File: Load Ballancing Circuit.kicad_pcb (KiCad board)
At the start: 2 copper layers, 39.4 x 46.6 mm, 12 parts, among them J1 1757284, U1 LTC4359HMS8#PBF, U2 LTC4359HMS8#PBF

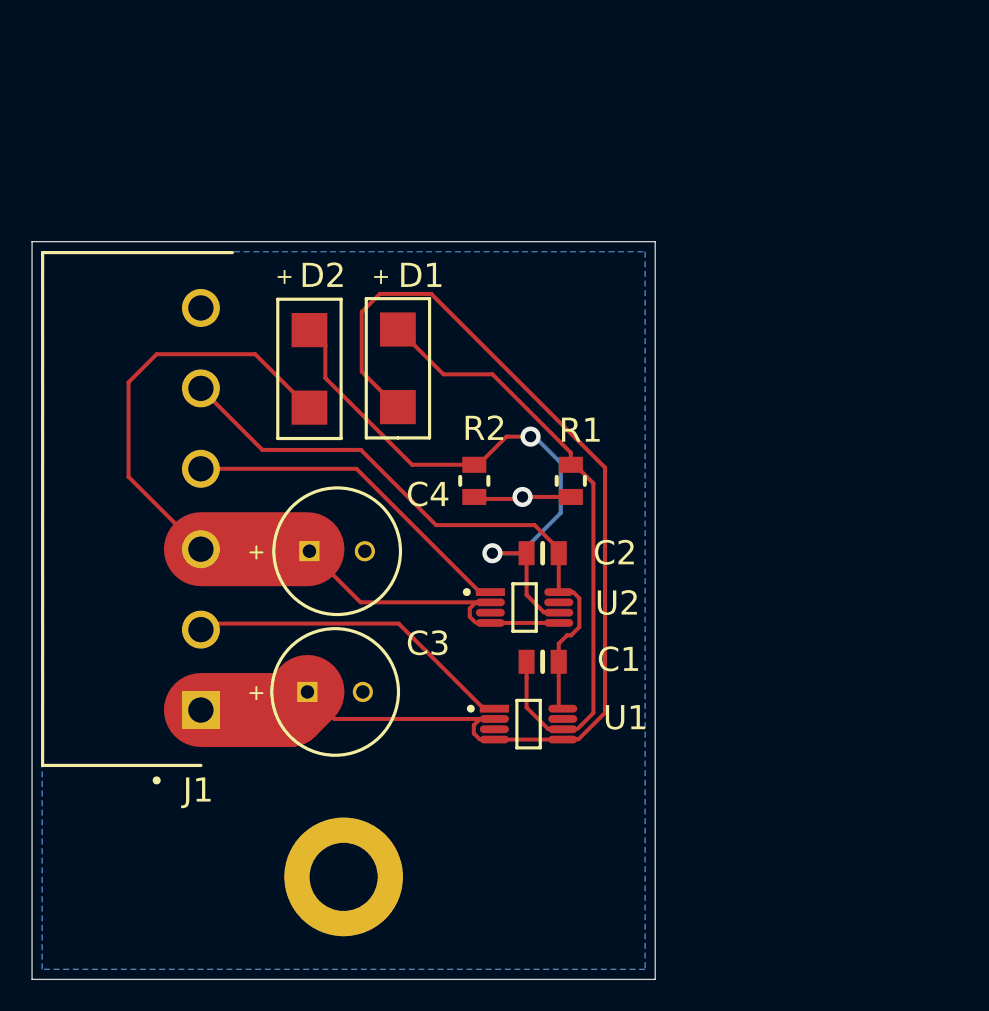
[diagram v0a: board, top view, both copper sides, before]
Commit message: added connectors and did layout
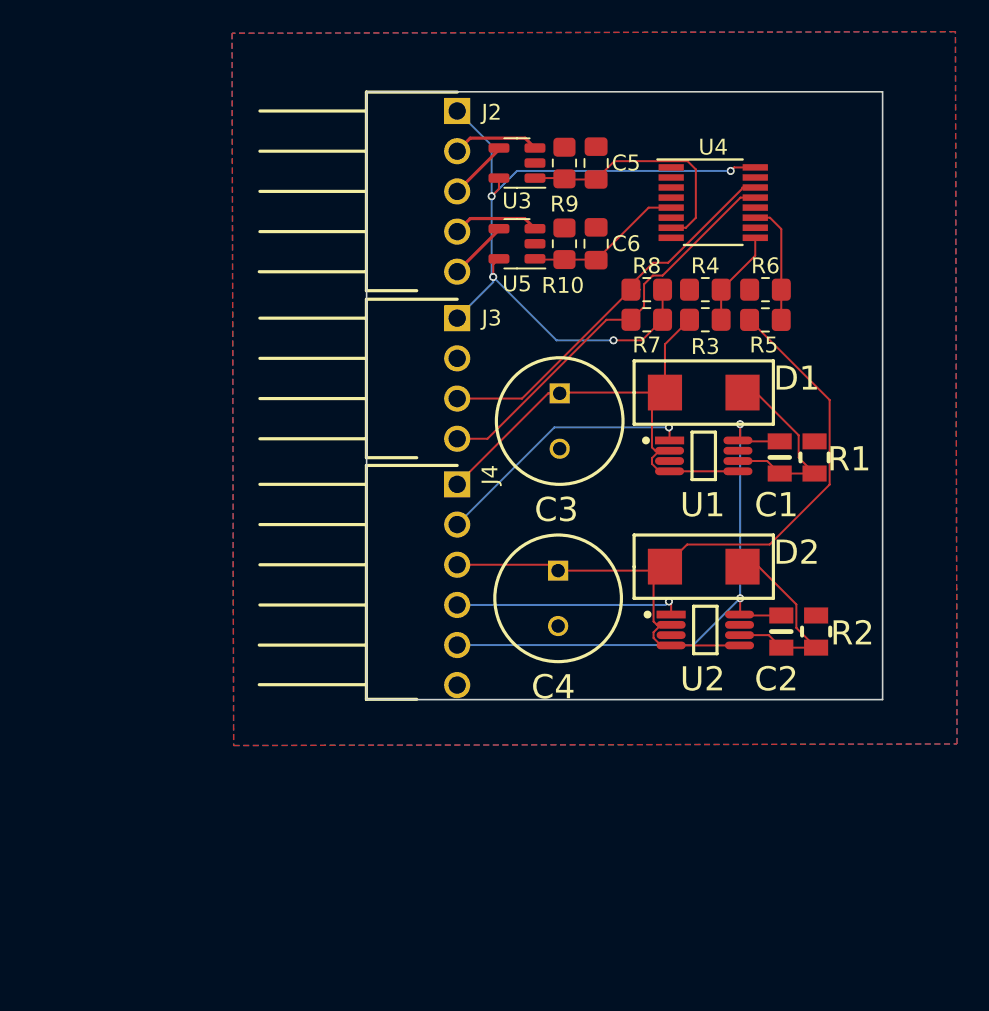
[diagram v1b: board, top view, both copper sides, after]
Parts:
- removed J1: 1757284, AltiumImport:SHDRRA6W100P0X508_1X6_3240X1200X860P
- removed REF**: MountingHole_4.3mm_M4_DIN965_Pad, AltiumImport:MountingHole_4.3mm_M4_DIN965_Pad
- added C5: 8p, Capacitor_SMD:C_0805_2012Metric_Pad1.18x1.45mm_HandSolder, F.Cu at (164.5, 76.7)
- added C6: 8p, Capacitor_SMD:C_0805_2012Metric_Pad1.18x1.45mm_HandSolder, F.Cu at (164.5, 81.8)
- added J2: 171857-0005, KK254:1718570005, F.Cu at (157.0, 72.0)
- added J3: 171857-0004, KK254:1718570004, F.Cu at (157.0, 85.1)
- added J4: 171857-0006, KK254:1718570006, F.Cu at (157.0, 95.6)
- added R10: 27k, Resistor_SMD:R_0805_2012Metric_Pad1.20x1.40mm_HandSolder, F.Cu at (162.5, 81.8)
- added R3: 10M, Resistor_SMD:R_0805_2012Metric_Pad1.20x1.40mm_HandSolder, F.Cu at (171.4, 86.6)
- added R4: 1.38M, Resistor_SMD:R_0805_2012Metric_Pad1.20x1.40mm_HandSolder, F.Cu at (171.4, 84.7)
- added R5: 10M, Resistor_SMD:R_0805_2012Metric_Pad1.20x1.40mm_HandSolder, F.Cu at (175.1, 86.6)
- added R6: 1.38M, Resistor_SMD:R_0805_2012Metric_Pad1.20x1.40mm_HandSolder, F.Cu at (175.2, 84.7)
- added R7: DNP, Resistor_SMD:R_0805_2012Metric_Pad1.20x1.40mm_HandSolder, F.Cu at (167.7, 86.6)
- added R8: DNP, Resistor_SMD:R_0805_2012Metric_Pad1.20x1.40mm_HandSolder, F.Cu at (167.7, 84.7)
- added R9: 27k, Resistor_SMD:R_0805_2012Metric_Pad1.20x1.40mm_HandSolder, F.Cu at (162.5, 76.7)
- added U3: INA139, Package_TO_SOT_SMD:SOT-23-5, F.Cu at (159.5, 76.7)
- added U4: MAX11615, Package_SO:QSOP-16_3.9x4.9mm_P0.635mm, F.Cu at (171.9, 79.2)
- added U5: INA139, Package_TO_SOT_SMD:SOT-23-5, F.Cu at (159.5, 81.8)
- moved D2 27.9 mm to (171.3, 102.2), turned to 0 degrees
- moved C3 24.7 mm to (162.2, 91.3), turned to -90 degrees
- moved R2 23.6 mm to (178.4, 106.3), turned to 180 degrees
- moved U1 20.2 mm to (171.3, 95.2)
- moved C1 19.8 mm to (176.1, 95.3), turned to 0 degrees
- moved D1 19.4 mm to (171.3, 91.2), turned to 0 degrees
- moved C2 15.9 mm to (176.2, 106.3), turned to 0 degrees
- moved C4 15.8 mm to (162.1, 102.5), turned to -90 degrees
- moved R1 15.5 mm to (178.3, 95.3), turned to 180 degrees
- moved U2 11.5 mm to (171.4, 106.2)
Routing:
- net 3V3: track 0.00 -> 49.8 mm, vias 0 -> 4
- net /V_BAT_IN_1: track 73.7 -> 33.1 mm
- net /I2C_SCL: track 0.00 -> 26.0 mm
- net /I2C_SDA: track 0.00 -> 25.9 mm
- net Net-(D1-2): track 38.5 -> 12.7 mm
- net Net-(D2-2): track 38.0 -> 12.8 mm, vias 2 -> 0
- net Net-(U4-AIN2): track 0.00 -> 15.8 mm
- net Net-(U4-AIN0): track 0.00 -> 10.0 mm
- net Net-(U4-AIN6): track 0.00 -> 7.68 mm
- net /GATE_2: track 21.5 -> 14.4 mm, vias 0 -> 1
- net Net-(U4-AIN4): track 0.00 -> 6.07 mm
- net /SNS2+: track 0.00 -> 5.52 mm
- net /SNS1+: track 0.00 -> 5.51 mm
- net GND: track 5.21 -> 0.00 mm, vias 1 -> 0
- net /GATE_1: track 20.9 -> 16.8 mm, vias 0 -> 1
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- added copper zone on F.Cu, net GND
- removed copper zone on B.Cu, net (none)
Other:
- board size 39.4 x 46.6 mm -> 32.6 x 38.4 mm
- board text removed: "+"
- board text removed: "Load Balancing Board v1.0"

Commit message: board is now now a weird size
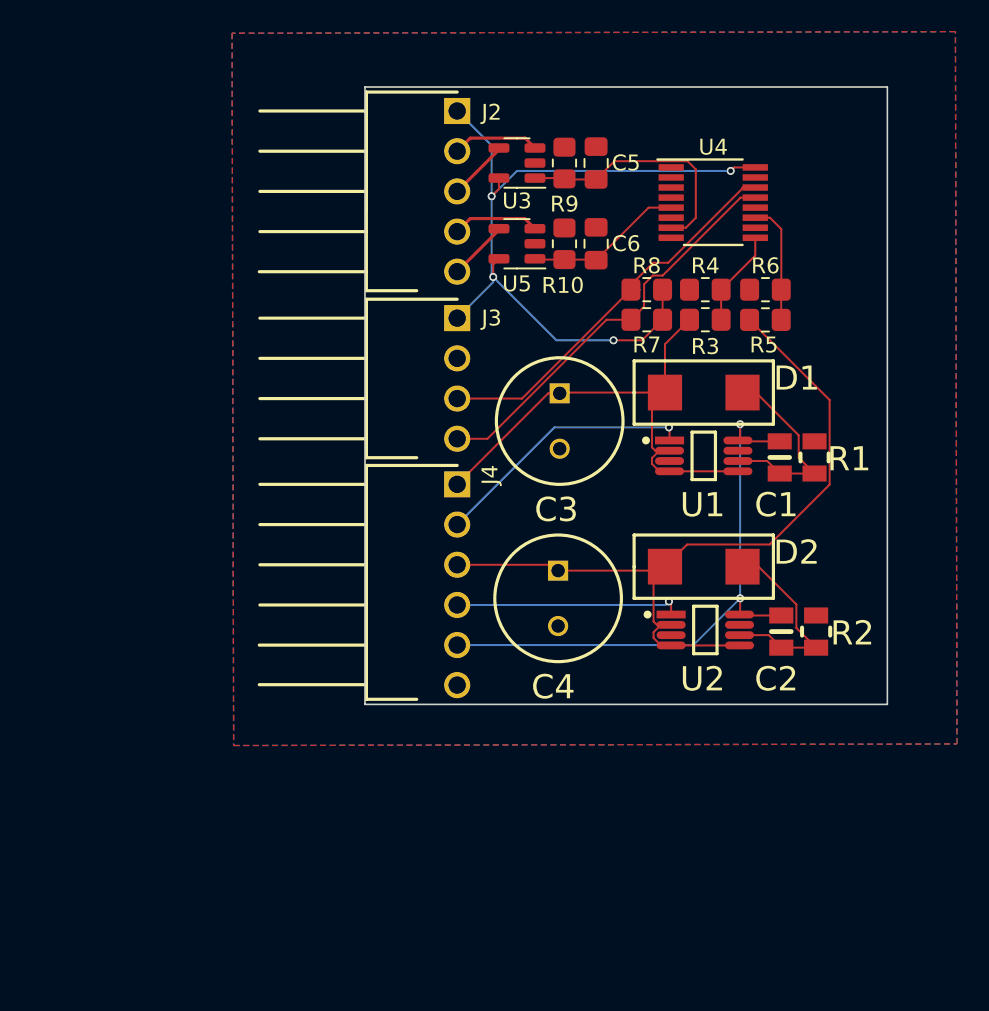
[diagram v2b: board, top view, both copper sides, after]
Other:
- board size 32.6 x 38.4 mm -> 33 x 39 mm
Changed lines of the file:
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@@
       (net 17 "/I2C_SCL") (pinfunction "4") (pintype "passive"))
   )
-  (gr_rect (start 149.9511 72.2331) (end 182.5511 110.6331)
+  (gr_rect (start 149.8511 71.9331) (end 182.8511 110.9331)
     (stroke (width 0.1016) (type default)) (fill none) (layer "Edge.Cuts"))
+  (dimension (type aligned) (layer "Edge.Cuts")
+    (pts (xy 182.8511 71.9331) (xy 149.8511 71.9331))
+    (height 5.5669)
+    (gr_text "33.0000 mm" (at 166.3511 65.2162) (layer "Edge.Cuts")
+      (effects (font (size 1 1) (thickness 0.15)))
+    )
+    (format (prefix "") (suffix "") (units 2) (units_format 1) (precision 4))
+    (style (thickness 0.1016) (arrow_length 1.27) (text_position_mode 0) (extension_height 0.58642) (extension_offset 0.508) keep_text_aligned)
+  )
+  (dimension (type aligned) (layer "Edge.Cuts")
+    (pts (xy 182.8511 110.9331) (xy 182.8511 71.9331))
+    (height 10.1)
+    (gr_text "39.0000 mm" (at 191.8011 91.4331 90) (layer "Edge.Cuts")
+      (effects (font (size 1 1) (thickness 0.15)))
+    )
+    (format (prefix "") (suffix "") (units 2) (units_format 1) (precision 4))
+    (style (thickness 0.1016) (arrow_length 1.27) (text_position_mode 0) (extension_height 0.58642) (extension_offset 0.508) keep_text_aligned)
+  )
   (segment (start 173.5511 105.21795) (end 173.51095 105.2581) (width 0.127) (layer "F.Cu") (net 1))
   (segment (start 173.51095 105.2581) (end 173.56995 105.3171) (width 0.127) (layer "F.Cu") (net 1))
